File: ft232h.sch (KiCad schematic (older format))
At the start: 14 parts, among them U3 93LCxxB, U4 FT232H, Y1 Crystal

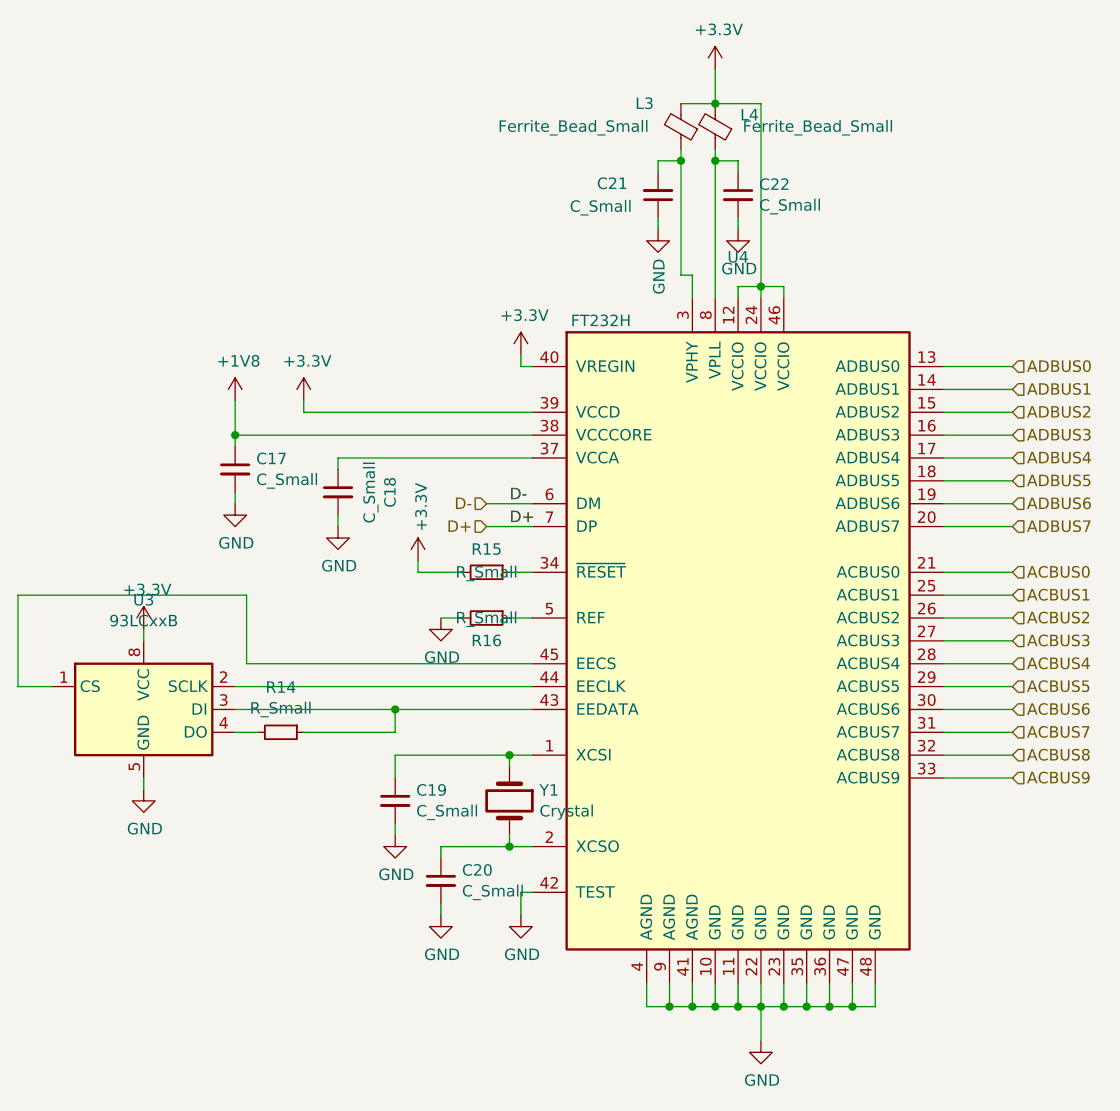
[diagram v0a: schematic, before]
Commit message: pcb updates or something
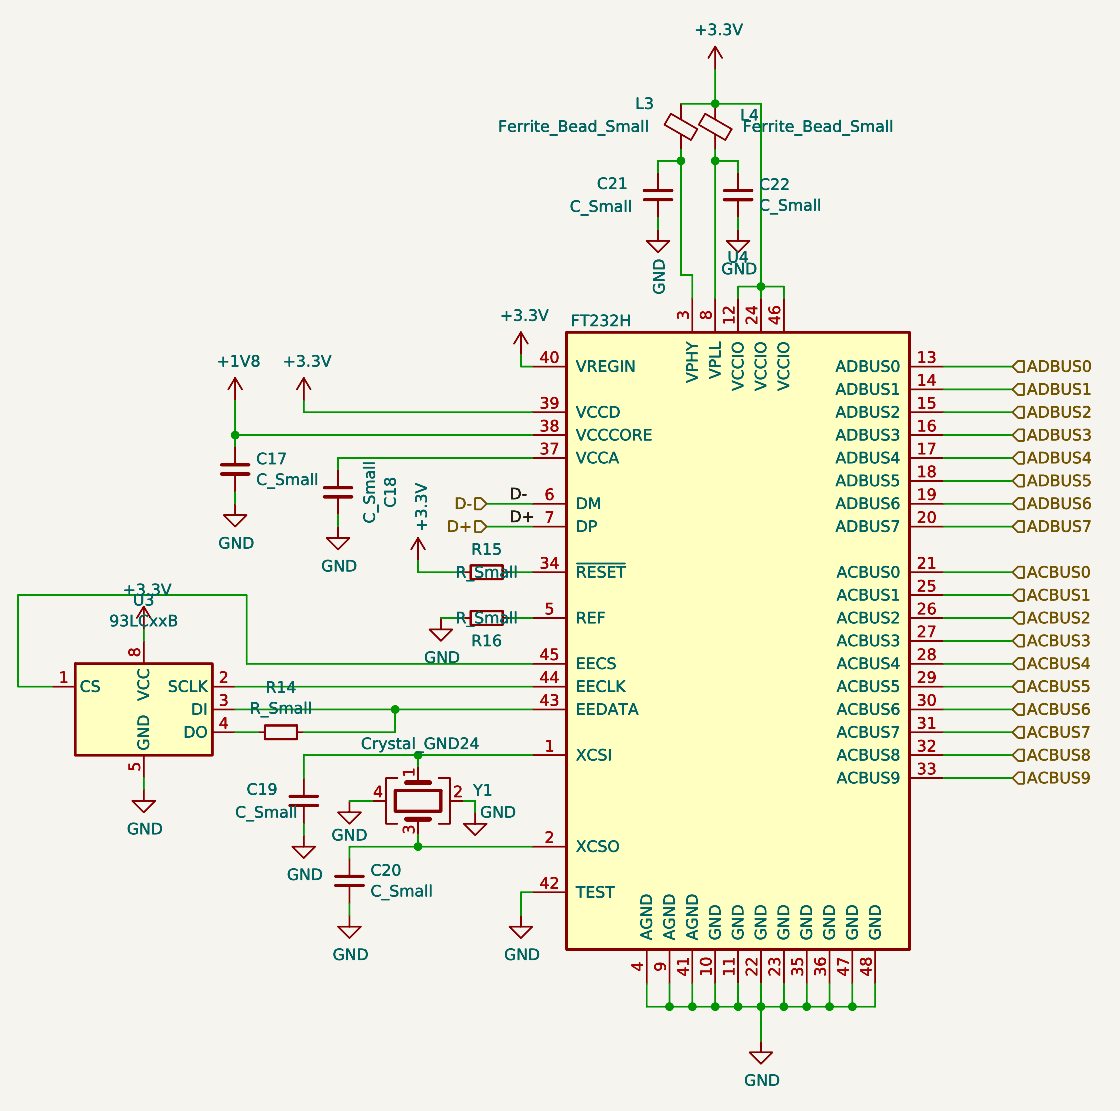
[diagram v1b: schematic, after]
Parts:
- removed Y1: Crystal, symbol Device:Crystal
- added Y1: Crystal_GND24, Crystals:Crystal_SMD_3225-4pin_3.2x2.5mm, symbol Device:Crystal_GND24
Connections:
- net GND: now also Y1.2, Y1.4
- net at C19.1, U4.1 (XCSI): now also Y1.1
- net at C20.1, U4.2 (XCSO): now also Y1.3
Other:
- moved on the sheet: C19, C20
